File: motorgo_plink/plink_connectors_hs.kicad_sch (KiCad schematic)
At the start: 11 parts, among them J13 I2C_STANDARDQWIIC, J14 BM05B-SRSS-TB_LF__SN_, J15 I2C_STANDARDQWIIC, J16 BM05B-SRSS-TB_LF__SN_, J18 BM05B-SRSS-TB_LF__SN_, J20 BM05B-SRSS-TB_LF__SN_, J5 Conn_02x20_Odd_Even

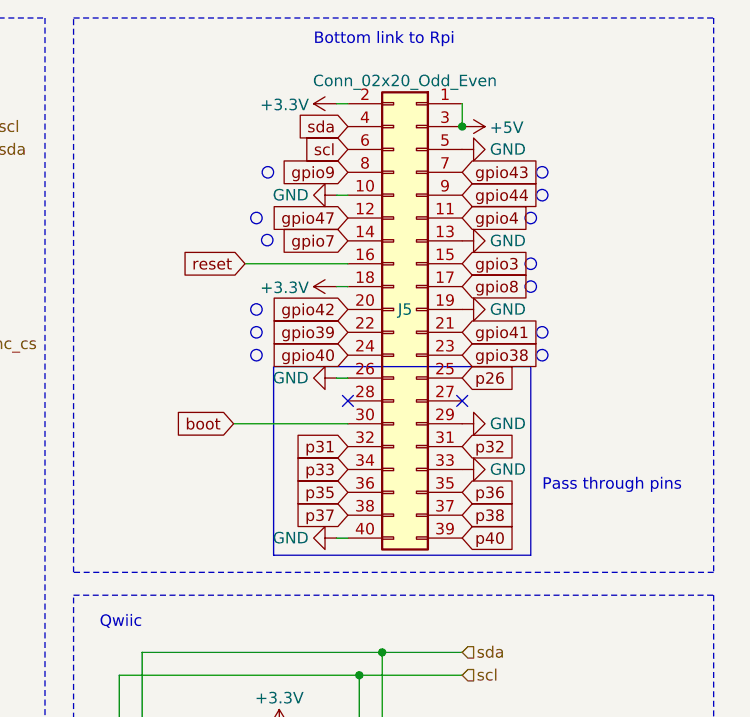
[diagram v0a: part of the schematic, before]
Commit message: layout complete! checkpoint ready for design review
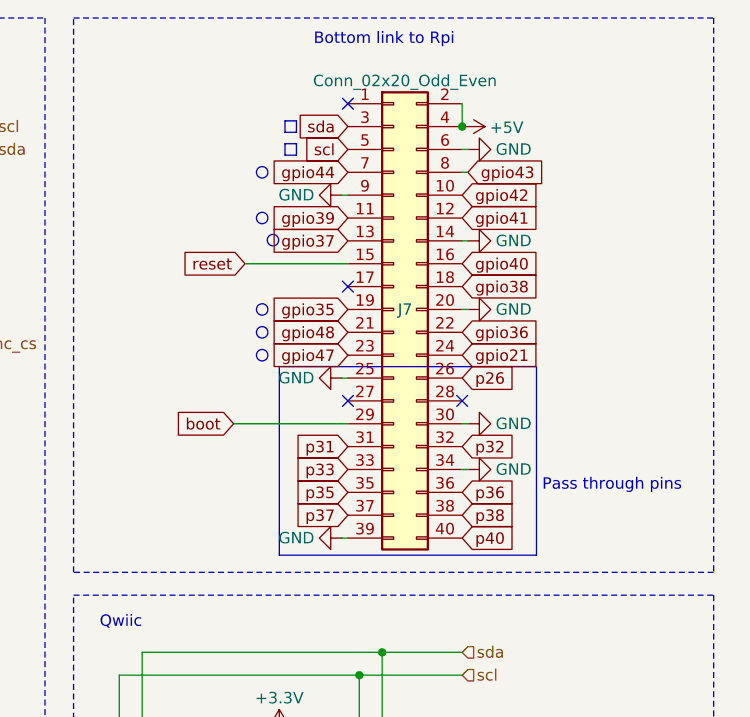
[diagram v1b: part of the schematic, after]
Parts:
- removed J5: Conn_02x20_Odd_Even, Connector_PinSocket_2.54mm:PinSocket_2x20_P2.54mm_Vertical_SMD, symbol Connector_Generic:Conn_02x20_Odd_Even
- added J7: Conn_02x20_Odd_Even, Connector_PinSocket_2.54mm:PinSocket_2x20_P2.54mm_Vertical_SMD, symbol Connector_Generic:Conn_02x20_Odd_Even
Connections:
- net +5V: now also J7.2 (Pin_2), J7.4 (Pin_4)
- net GND: now also J7.14 (Pin_14), J7.20 (Pin_20), J7.25 (Pin_25), J7.30 (Pin_30), J7.34 (Pin_34), J7.39 (Pin_39), J7.6 (Pin_6), J7.9 (Pin_9)
- net boot: now also J7.29 (Pin_29)
- net gpio38: now also J7.18 (Pin_18)
- net gpio39: now also J7.11 (Pin_11)
- net gpio40: now also J7.16 (Pin_16)
- net gpio41: now also J7.12 (Pin_12)
- net gpio42: now also J7.10 (Pin_10)
- net gpio43: now also J7.8 (Pin_8)
- net gpio44: now also J7.7 (Pin_7)
- net gpio47: now also J7.23 (Pin_23)
- net p26: now also J7.26 (Pin_26)
- net p31: now also J7.31 (Pin_31)
- net p32: now also J7.32 (Pin_32)
- net p33: now also J7.33 (Pin_33)
- net p35: now also J7.35 (Pin_35)
- net p36: now also J7.36 (Pin_36)
- net p37: now also J7.37 (Pin_37)
- net p38: now also J7.38 (Pin_38)
- net p40: now also J7.40 (Pin_40)
- net reset: now also J7.15 (Pin_15)
- net scl: now also J7.5 (Pin_5)
- net sda: now also J7.3 (Pin_3)
- new net gpio21: J7.24 (Pin_24)
- new net gpio35: J7.19 (Pin_19)
- new net gpio36: J7.22 (Pin_22)
- new net gpio37: J7.13 (Pin_13)
- new net gpio48: J7.21 (Pin_21)
- no-connect marks 2 -> 4

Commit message: production files and all edits for final send off of v1.0
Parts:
- R30, R31, R32, R33: LCSC_Part_Number C409700 -> C25905
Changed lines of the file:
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@@
 			)
 		)
-		(property "LCSC_Part_Number" "C409700"
+		(property "LCSC_Part_Number" "C25905"
 			(at 95.25 49.53 0)
 			(effects
@@
 			)
 		)
-		(property "LCSC_Part_Number" "C409700"
+		(property "LCSC_Part_Number" "C25905"
 			(at 187.96 105.41 0)
 			(effects
@@
 			)
 		)
-		(property "LCSC_Part_Number" "C409700"
+		(property "LCSC_Part_Number" "C25905"
 			(at 185.42 105.41 0)
 			(effects
@@
 			)
 		)
-		(property "LCSC_Part_Number" "C409700"
+		(property "LCSC_Part_Number" "C25905"
 			(at 97.79 49.53 0)
 			(effects
